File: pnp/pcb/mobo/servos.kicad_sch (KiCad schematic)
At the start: 2 parts, among them J15 SERVO1, J16 SERVO2

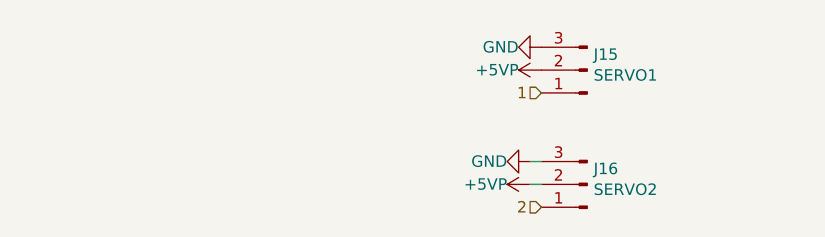
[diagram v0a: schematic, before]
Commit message: replaces SRL05 for SRV05 due to pricing and availability, routed mostfet gate resistors and added 2g34 buffer to boost the voltage of the servo drive pins. consolidated a random cap value that could be switched to an existing one.
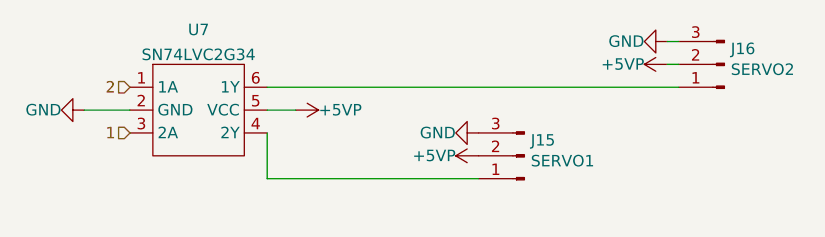
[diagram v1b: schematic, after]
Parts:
- added U7: SN74LVC2G34, Package_TO_SOT_SMD:SOT-23-6, symbol index:SN74LVC2G34
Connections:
- net +5VP: now also U7.5 (VCC)
- net 1: now also U7.3 (2A); no longer J15.1 (Pin_1)
- net 2: now also U7.1 (1A); no longer J16.1 (Pin_1)
- net GND: now also U7.2 (GND)
- new net: J15.1 (Pin_1), U7.4 (2Y)
- new net: J16.1 (Pin_1), U7.6 (1Y)
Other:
- moved on the sheet: J15, J16
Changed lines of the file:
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@@
     (company "Opulo")
   )
-  (wire (pts (xy 148.59 106.68) (xy 149.86 106.68))
+  (wire (pts (xy 119.38 108.585) (xy 142.875 108.585))
     (stroke (width 0) (type default) (color 0 0 0 0))
   )
-  (wire (pts (xy 148.59 109.22) (xy 149.86 109.22))
+  (wire (pts (xy 163.83 93.345) (xy 165.1 93.345))
     (stroke (width 0) (type default) (color 0 0 0 0))
   )
-  (hierarchical_label "1" (shape input) (at 149.86 99.06 180)
+  (wire (pts (xy 119.38 108.585) (xy 119.38 103.505))
+    (stroke (width 0) (type default) (color 0 0 0 0))
+  )
+  (wire (pts (xy 163.83 95.885) (xy 165.1 95.885))
+    (stroke (width 0) (type default) (color 0 0 0 0))
+  )
+  (wire (pts (xy 119.38 100.965) (xy 122.555 100.965))
+    (stroke (width 0) (type default) (color 0 0 0 0))
+  )
+  (wire (pts (xy 119.38 98.425) (xy 165.1 98.425))
+    (stroke (width 0) (type default) (color 0 0 0 0))
+  )
+  (wire (pts (xy 99.06 100.965) (xy 104.14 100.965))
+    (stroke (width 0) (type default) (color 0 0 0 0))
+  )
+  (hierarchical_label "1" (shape input) (at 104.14 103.505 180)
     (effects (font (size 1.27 1.27)) (justify right))
   )
-  (hierarchical_label "2" (shape input) (at 149.86 111.76 180)
+  (hierarchical_label "2" (shape input) (at 104.14 98.425 180)
     (effects (font (size 1.27 1.27)) (justify right))
   )
-  (symbol (lib_id "power:+5VP") (at 149.86 96.52 90) (unit 1)
+  (symbol (lib_id "power:+5VP") (at 142.875 106.045 90) (unit 1)
     (in_bom yes) (on_board yes)
-    (property "Reference" "#PWR0171" (id 0) (at 153.67 96.52 0)
+    (property "Reference" "#PWR0171" (id 0) (at 146.685 106.045 0)
       (effects (font (size 1.27 1.27)) hide)
     )
-    (property "Value" "+5VP" (id 1) (at 147.32 96.52 90)
+    (property "Value" "+5VP" (id 1) (at 140.335 106.045 90)
       (effects (font (size 1.27 1.27)) (justify left))
     )
-    (property "Footprint" "" (id 2) (at 149.86 96.52 0)
+    (property "Footprint" "" (id 2) (at 142.875 106.045 0)
       (effects (font (size 1.27 1.27)) hide)
     )
-    (property "Datasheet" "" (id 3) (at 149.86 96.52 0)
+    (property "Datasheet" "" (id 3) (at 142.875 106.045 0)
       (effects (font (size 1.27 1.27)) hide)
     )
     (pin "1")
   )
-  (symbol (lib_id "power:GND") (at 149.86 93.98 270) (unit 1)
-    (in_bom yes) (on_board yes)
-    (property "Reference" "#PWR0170" (id 0) (at 143.51 93.98 0)
+  (symbol (lib_id "index:SN74LVC2G34") (at 111.76 106.045 0) (unit 1)
+    (in_bom yes) (on_board yes) (fields_autoplaced)
+    (property "Reference" "U7" (id 0) (at 111.76 92.0455 0))
+    (property "Value" "SN74LVC2G34" (id 1) (at 111.76 94.8206 0))
+    (property "Footprint" "Package_TO_SOT_SMD:SOT-23-6" (id 2) (at 111.76 106.045 0)
       (effects (font (size 1.27 1.27)) hide)
     )
-    (property "Value" "GND" (id 1) (at 147.32 93.98 90)
+    (property "Datasheet" "https://www.ti.com/cn/lit/ds/symlink/sn74lvc2g34.pdf?ts=1659406501708" (id 3) (at 111.76 106.045 0)
+      (effects (font (size 1.27 1.27)) hide)
+    )
+    (pin "1")
+    (pin "2")
+    (pin "3")
+    (pin "4")
+    (pin "5")
+    (pin "6")
+  )
+  (symbol (lib_id "power:GND") (at 142.875 103.505 270) (unit 1)
+    (in_bom yes) (on_board yes)
+    (property "Reference" "#PWR0170" (id 0) (at 136.525 103.505 0)
+      (effects (font (size 1.27 1.27)) hide)
+    )
+    (property "Value" "GND" (id 1) (at 140.335 103.505 90)
       (effects (font (size 1.27 1.27)) (justify right))
     )
-    (property "Footprint" "" (id 2) (at 149.86 93.98 0)
+    (property "Footprint" "" (id 2) (at 142.875 103.505 0)
       (effects (font (size 1.27 1.27)) hide)
     )
-    (property "Datasheet" "" (id 3) (at 149.86 93.98 0)
+    (property "Datasheet" "" (id 3) (at 142.875 103.505 0)
       (effects (font (size 1.27 1.27)) hide)
     )
     (pin "1")
   )
-  (symbol (lib_id "power:GND") (at 148.59 106.68 270) (unit 1)
+  (symbol (lib_id "power:GND") (at 99.06 100.965 270) (unit 1)
     (in_bom yes) (on_board yes)
-    (property "Reference" "#PWR0172" (id 0) (at 142.24 106.68 0)
+    (property "Reference" "#PWR0137" (id 0) (at 92.71 100.965 0)
       (effects (font (size 1.27 1.27)) hide)
     )
-    (property "Value" "GND" (id 1) (at 146.05 106.68 90)
+    (property "Value" "GND" (id 1) (at 96.52 100.965 90)
       (effects (font (size 1.27 1.27)) (justify right))
     )
-    (property "Footprint" "" (id 2) (at 148.59 106.68 0)
+    (property "Footprint" "" (id 2) (at 99.06 100.965 0)
       (effects (font (size 1.27 1.27)) hide)
     )
-    (property "Datasheet" "" (id 3) (at 148.59 106.68 0)
+    (property "Datasheet" "" (id 3) (at 99.06 100.965 0)
       (effects (font (size 1.27 1.27)) hide)
     )
     (pin "1")
   )
-  (symbol (lib_id "power:+5VP") (at 148.59 109.22 90) (unit 1)
+  (symbol (lib_id "power:GND") (at 163.83 93.345 270) (unit 1)
     (in_bom yes) (on_board yes)
-    (property "Reference" "#PWR0173" (id 0) (at 152.4 109.22 0)
+    (property "Reference" "#PWR0172" (id 0) (at 157.48 93.345 0)
       (effects (font (size 1.27 1.27)) hide)
     )
-    (property "Value" "+5VP" (id 1) (at 146.05 109.22 90)
-      (effects (font (size 1.27 1.27)) (justify left))
+    (property "Value" "GND" (id 1) (at 161.29 93.345 90)
+      (effects (font (size 1.27 1.27)) (justify right))
     )
-    (property "Footprint" "" (id 2) (at 148.59 109.22 0)
+    (property "Footprint" "" (id 2) (at 163.83 93.345 0)
       (effects (font (size 1.27 1.27)) hide)
     )
-    (property "Datasheet" "" (id 3) (at 148.59 109.22 0)
+    (property "Datasheet" "" (id 3) (at 163.83 93.345 0)
       (effects (font (size 1.27 1.27)) hide)
     )
     (pin "1")
   )
-  (symbol (lib_id "Connector:Conn_01x03_Male") (at 154.94 96.52 180) (unit 1)
+  (symbol (lib_id "power:+5VP") (at 163.83 95.885 90) (unit 1)
     (in_bom yes) (on_board yes)
-    (property "Reference" "J15" (id 0) (at 155.6512 94.7928 0)
+    (property "Reference" "#PWR0173" (id 0) (at 167.64 95.885 0)
+      (effects (font (size 1.27 1.27)) hide)
+    )
+    (property "Value" "+5VP" (id 1) (at 161.29 95.885 90)
+      (effects (font (size 1.27 1.27)) (justify left))
+    )
+    (property "Footprint" "" (id 2) (at 163.83 95.885 0)
+      (effects (font (size 1.27 1.27)) hide)
+    )
+    (property "Datasheet" "" (id 3) (at 163.83 95.885 0)
+      (effects (font (size 1.27 1.27)) hide)
+    )
+    (pin "1")
+  )
+  (symbol (lib_id "Connector:Conn_01x03_Male") (at 147.955 106.045 180) (unit 1)
+    (in_bom yes) (on_board yes)
+    (property "Reference" "J15" (id 0) (at 148.6662 104.3178 0)
       (effects (font (size 1.27 1.27)) (justify right))
     )
-    (property "Value" "SERVO1" (id 1) (at 155.6512 97.1042 0)
+    (property "Value" "SERVO1" (id 1) (at 148.6662 106.6292 0)
       (effects (font (size 1.27 1.27)) (justify right))
     )
-    (property "Footprint" "Connector_JST:JST_XH_B3B-XH-A_1x03_P2.50mm_Vertical" (id 2) (at 154.94 96.52 0)
+    (property "Footprint" "Connector_JST:JST_XH_B3B-XH-A_1x03_P2.50mm_Vertical" (id 2) (at 147.955 106.045 0)
       (effects (font (size 1.27 1.27)) hide)
     )
-    (property "Datasheet" "" (id 3) (at 154.94 96.52 0)
+    (property "Datasheet" "" (id 3) (at 147.955 106.045 0)
       (effects (font (size 1.27 1.27)) hide)
     )
-    (property "LCSC" "C2316" (id 4) (at 154.94 96.52 0)
+    (property "LCSC" "C2316" (id 4) (at 147.955 106.045 0)
       (effects (font (size 1.27 1.27)) hide)
     )
-    (property "JLCPCB" "C2316" (id 5) (at 154.94 96.52 0)
+    (property "JLCPCB" "C2316" (id 5) (at 147.955 106.045 0)
       (effects (font (size 1.27 1.27)) hide)
     )
-    (property "Digikey" "455-2248-ND" (id 6) (at 154.94 96.52 0)
+    (property "Digikey" "455-2248-ND" (id 6) (at 147.955 106.045 0)
       (effects (font (size 1.27 1.27)) hide)
     )
@@
     (pin "3")
   )
-  (symbol (lib_id "Connector:Conn_01x03_Male") (at 154.94 109.22 180) (unit 1)
+  (symbol (lib_id "power:+5VP") (at 122.555 100.965 270) (unit 1)
     (in_bom yes) (on_board yes)
-    (property "Reference" "J16" (id 0) (at 155.6512 107.4928 0)
+    (property "Reference" "#PWR0134" (id 0) (at 118.745 100.965 0)
+      (effects (font (size 1.27 1.27)) hide)
+    )
+    (property "Value" "+5VP" (id 1) (at 125.095 100.965 90)
+      (effects (font (size 1.27 1.27)) (justify left))
+    )
+    (property "Footprint" "" (id 2) (at 122.555 100.965 0)
+      (effects (font (size 1.27 1.27)) hide)
+    )
+    (property "Datasheet" "" (id 3) (at 122.555 100.965 0)
+      (effects (font (size 1.27 1.27)) hide)
+    )
+    (pin "1")
+  )
+  (symbol (lib_id "Connector:Conn_01x03_Male") (at 170.18 95.885 180) (unit 1)
+    (in_bom yes) (on_board yes)
+    (property "Reference" "J16" (id 0) (at 170.8912 94.1578 0)
       (effects (font (size 1.27 1.27)) (justify right))
     )
-    (property "Value" "SERVO2" (id 1) (at 155.6512 109.8042 0)
+    (property "Value" "SERVO2" (id 1) (at 170.8912 96.4692 0)
       (effects (font (size 1.27 1.27)) (justify right))
     )
-    (property "Footprint" "Connector_JST:JST_XH_B3B-XH-A_1x03_P2.50mm_Vertical" (id 2) (at 154.94 109.22 0)
+    (property "Footprint" "Connector_JST:JST_XH_B3B-XH-A_1x03_P2.50mm_Vertical" (id 2) (at 170.18 95.885 0)
       (effects (font (size 1.27 1.27)) hide)
     )
-    (property "Datasheet" "" (id 3) (at 154.94 109.22 0)
+    (property "Datasheet" "" (id 3) (at 170.18 95.885 0)
       (effects (font (size 1.27 1.27)) hide)
     )
-    (property "LCSC" "C2316" (id 4) (at 154.94 109.22 0)
+    (property "LCSC" "C2316" (id 4) (at 170.18 95.885 0)
       (effects (font (size 1.27 1.27)) hide)
     )
-    (property "JLCPCB" "C2316" (id 5) (at 154.94 109.22 0)
+    (property "JLCPCB" "C2316" (id 5) (at 170.18 95.885 0)
       (effects (font (size 1.27 1.27)) hide)
     )
-    (property "Digikey" "455-2248-ND" (id 6) (at 154.94 109.22 0)
+    (property "Digikey" "455-2248-ND" (id 6) (at 170.18 95.885 0)
       (effects (font (size 1.27 1.27)) hide)
     )

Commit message: Update mobo schematic with part numbers and ratings
All parts now have part numbers for at least one reseller or manufacturer along with rating specifications.

Note: I did not update the PCB with these new properties, as it seems the PCB is a bit out of sync with the schematic.
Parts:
- U7: Digikey (none) -> SN74LVC2G34DBVR
